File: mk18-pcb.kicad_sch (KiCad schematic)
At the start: 88 parts, among them J10 Conn_02x07_Top_Bottom, J17 Conn_01x06_Socket, J18 Conn_01x06_Socket, J19 Conn_01x06_Socket, J20 Conn_01x06_Socket, J7 Conn_02x06_Top_Bottom, J8 Conn_02x07_Top_Bottom, J9 Conn_02x06_Top_Bottom, P1 FH26W-13S-0_3SHW(60), P10 FH26W-13S-0_3SHW(60), P11 FH26W-13S-0_3SHW(60), P2 FH26W-13S-0_3SHW(60), P3 FH26W-13S-0_3SHW(60), P4 FH26W-13S-0_3SHW(60), P5 FH26W-13S-0_3SHW(60), P6 FH26W-13S-0_3SHW(60), P7 FH26W-13S-0_3SHW(60), P8 FH26W-13S-0_3SHW(60), P9 FH26W-13S-0_3SHW(60), U1 TYPE-C-31-M-12, U10 1N4148W_C81598, U11 1N4148W_C81598, U12 1N4148W_C81598, U13 1N4148W_C81598, U14 1N4148W_C81598, U15 1N4148W_C81598, U16 ECT818001569, U17 HC-FPC-05-10-16RLTAG, U2 AZC199-04S-MS, U3 1N4148W_C81598, U4 1N4148W_C81598, U4 SN74LVC1T45DRL, U5 1N4148W_C81598, U6 1N4148W_C81598, U7 1N4148W_C81598, U9 1N4148W_C81598

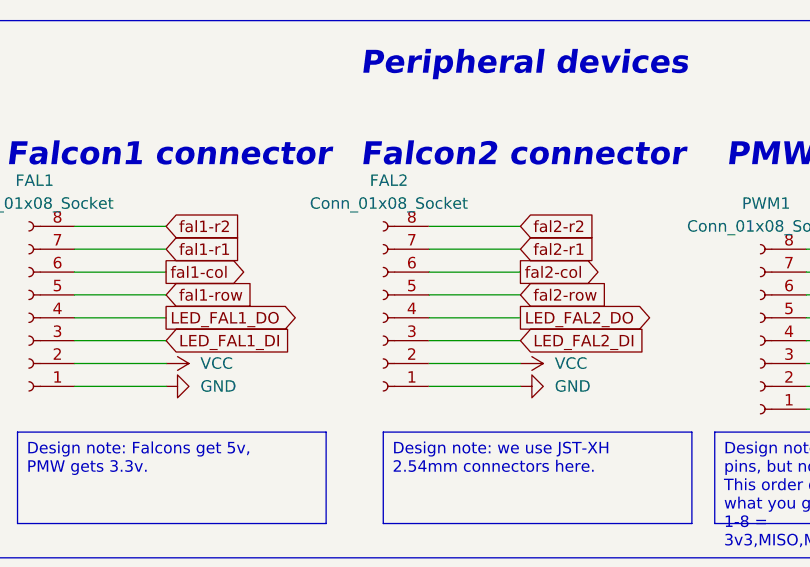
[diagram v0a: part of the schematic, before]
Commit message: really close now maybe kinda
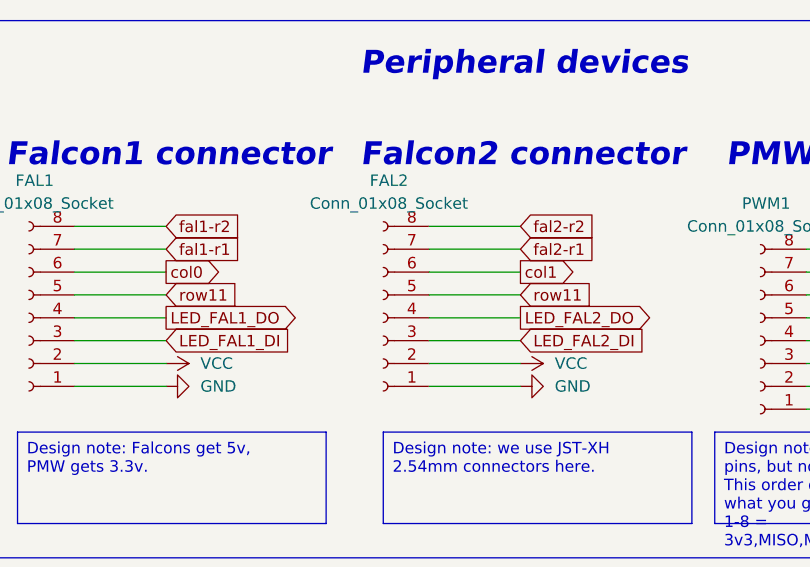
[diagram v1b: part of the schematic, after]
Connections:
- net col0: now also FAL1.6 (Pin_6)
- net col1: now also FAL2.6 (Pin_6)
- net fal1-col: no longer FAL1.6 (Pin_6)
- net fal1-row: no longer FAL1.5 (Pin_5)
- net fal2-col: no longer FAL2.6 (Pin_6)
- net fal2-row: no longer FAL2.5 (Pin_5)
- net row11: now also FAL1.5 (Pin_5), FAL2.5 (Pin_5)
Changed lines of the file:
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@@
     )
   )
-  (global_label "fal1-row" (shape input) (at 224.79 93.98 0) (fields_autoplaced)
-    (effects (font (size 1.27 1.27)) (justify left))
-    (property "Intersheetrefs" "${INTERSHEET_REFS}" (at 236.3627 93.98 0)
+  (global_label "row11" (shape input) (at 224.79 93.98 0) (fields_autoplaced)
+    (effects (font (size 1.27 1.27)) (justify left))
+    (property "Intersheetrefs" "${INTERSHEET_REFS}" (at 233.4599 93.98 0)
       (effects (font (size 1.27 1.27)) (justify left) hide)
     )
@@
     )
   )
-  (global_label "fal1-col" (shape output) (at 224.79 91.44 0) (fields_autoplaced)
-    (effects (font (size 1.27 1.27)) (justify left))
-    (property "Intersheetrefs" "${INTERSHEET_REFS}" (at 235.9998 91.44 0)
+  (global_label "col0" (shape output) (at 224.79 91.44 0) (fields_autoplaced)
+    (effects (font (size 1.27 1.27)) (justify left))
+    (property "Intersheetrefs" "${INTERSHEET_REFS}" (at 231.8875 91.44 0)
       (effects (font (size 1.27 1.27)) (justify left) hide)
     )
@@
     )
   )
-  (global_label "fal2-row" (shape input) (at 264.16 93.98 0) (fields_autoplaced)
-    (effects (font (size 1.27 1.27)) (justify left))
-    (property "Intersheetrefs" "${INTERSHEET_REFS}" (at 275.7327 93.98 0)
+  (global_label "row11" (shape input) (at 264.16 93.98 0) (fields_autoplaced)
+    (effects (font (size 1.27 1.27)) (justify left))
+    (property "Intersheetrefs" "${INTERSHEET_REFS}" (at 272.8299 93.98 0)
       (effects (font (size 1.27 1.27)) (justify left) hide)
     )
@@
     )
   )
-  (global_label "fal2-col" (shape output) (at 264.16 91.44 0) (fields_autoplaced)
-    (effects (font (size 1.27 1.27)) (justify left))
-    (property "Intersheetrefs" "${INTERSHEET_REFS}" (at 275.3698 91.44 0)
-      (effects (font (size 1.27 1.27)) (justify left) hide)
-    )
+  (global_label "col1" (shape output) (at 264.16 91.44 0) (fields_autoplaced)
+    (effects (font (size 1.27 1.27)) (justify left))
+    (property "Intersheetrefs" "${INTERSHEET_REFS}" (at 271.2575 91.44 0)
+      (effects (font (size 1.27 1.27)) (justify left) hide)
+    )

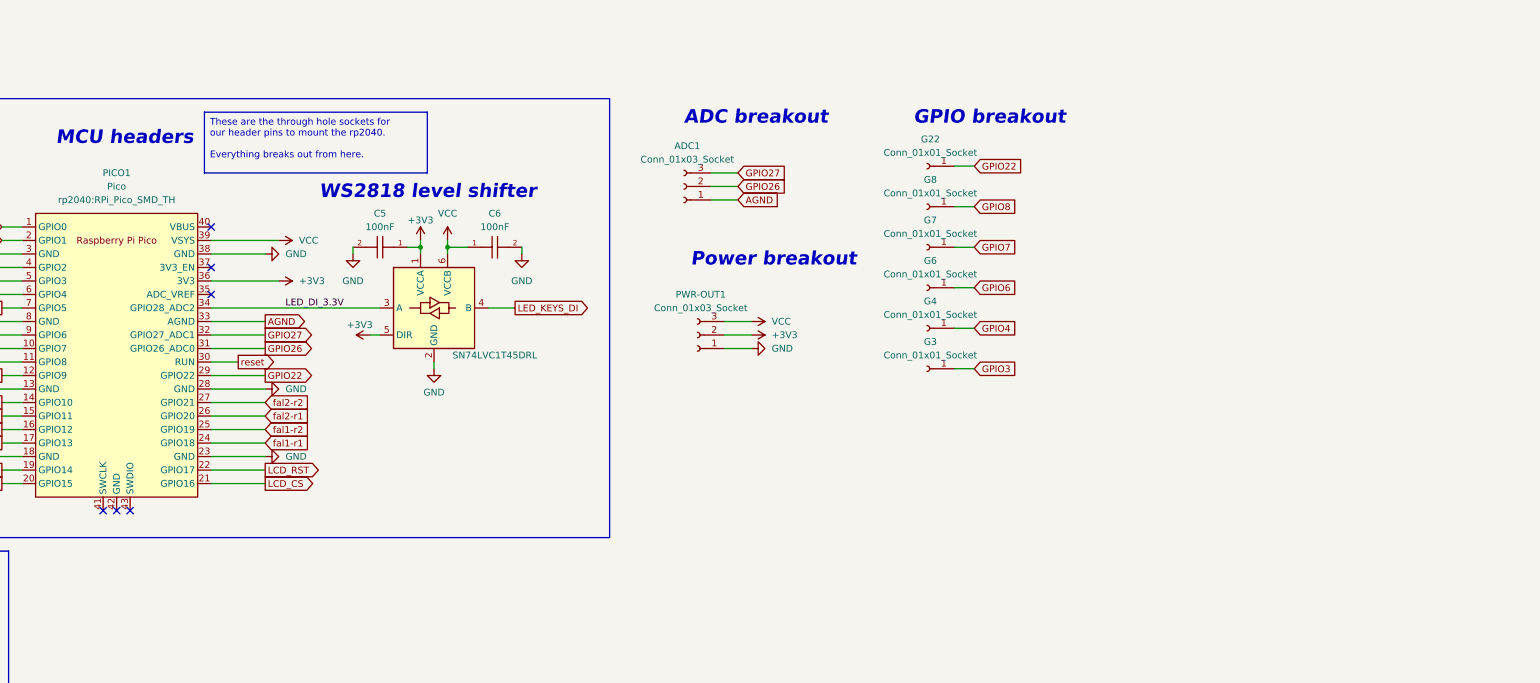
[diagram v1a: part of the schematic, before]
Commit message: added debug, test points, more
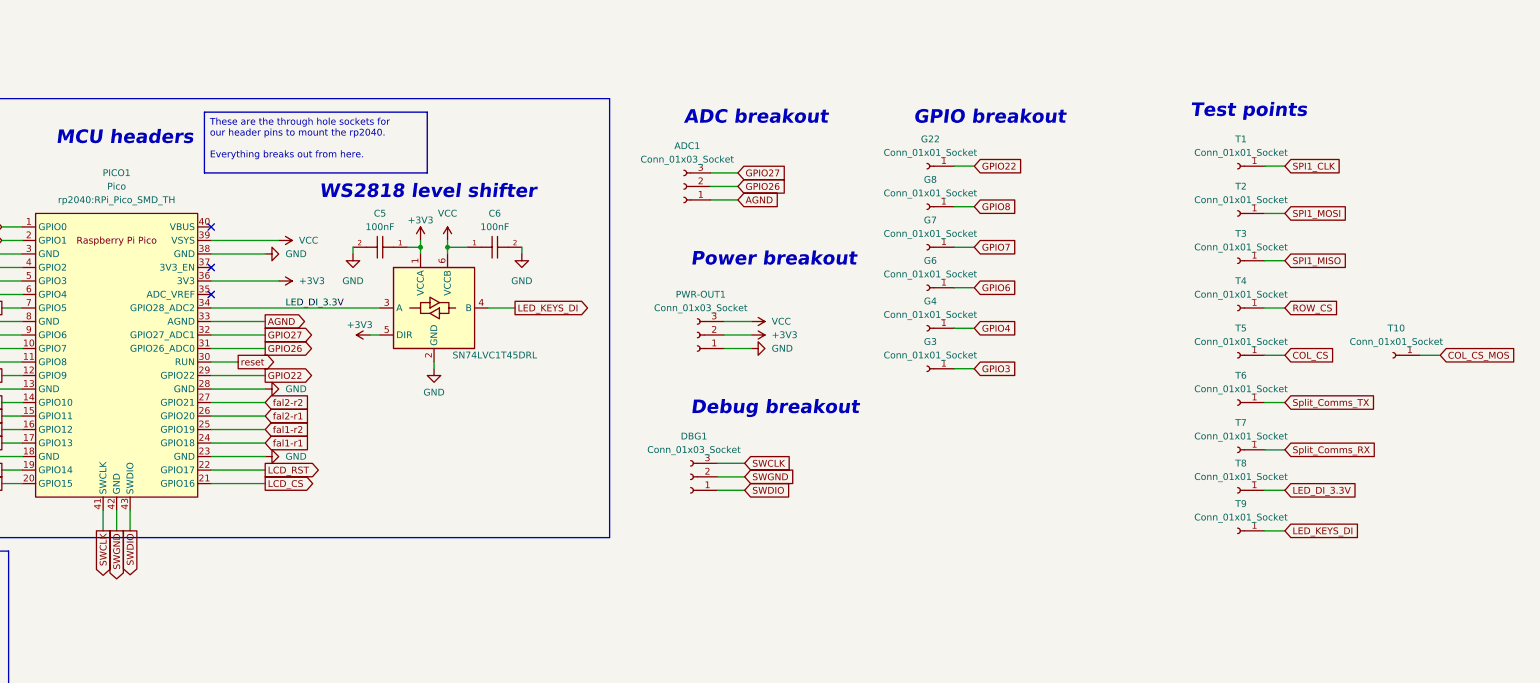
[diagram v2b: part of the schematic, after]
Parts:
- added DBG1: Conn_01x03_Socket, Connector_JST:JST_EH_B3B-EH-A_1x03_P2.50mm_Vertical, symbol Connector:Conn_01x03_Socket
- added T1, T10, T2, T3, T4, T5, T6, T7, T8, T9: Conn_01x01_Socket, Connector_Pin:Pin_D1.0mm_L10.0mm, symbol Connector:Conn_01x01_Socket
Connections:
- net COL_CS: now also T5.1 (Pin_1)
- net COL_CS_MOS: now also T10.1 (Pin_1)
- net LED_DI_3.3V: now also T8.1 (Pin_1)
- net LED_KEYS_DI: now also T9.1 (Pin_1)
- net ROW_CS: now also T4.1 (Pin_1)
- net SPI1_CLK: now also T1.1 (Pin_1)
- net SPI1_MISO: now also T3.1 (Pin_1)
- net SPI1_MOSI: now also T2.1 (Pin_1)
- net Split_Comms_RX: now also T7.1 (Pin_1)
- net Split_Comms_TX: now also T6.1 (Pin_1)
- net SWCLK: now reaches PICO1.41 (SWCLK)
- net SWCLK: now also DBG1.3 (Pin_3)
- net SWGND: now reaches PICO1.42 (GND)
- net SWGND: now also DBG1.2 (Pin_2)
- net SWDIO: now reaches PICO1.43 (SWDIO)
- net SWDIO: now also DBG1.1 (Pin_1)
- no-connect marks 34 -> 31
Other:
- note added: "Debug breakout"
- note added: "Test points"
